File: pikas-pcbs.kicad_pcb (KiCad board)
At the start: 2 copper layers, 84.1 x 43.7 mm, 24 parts, among them SW1 SW_Push, U1 ATmega32U4-AU, Y1 16MHz

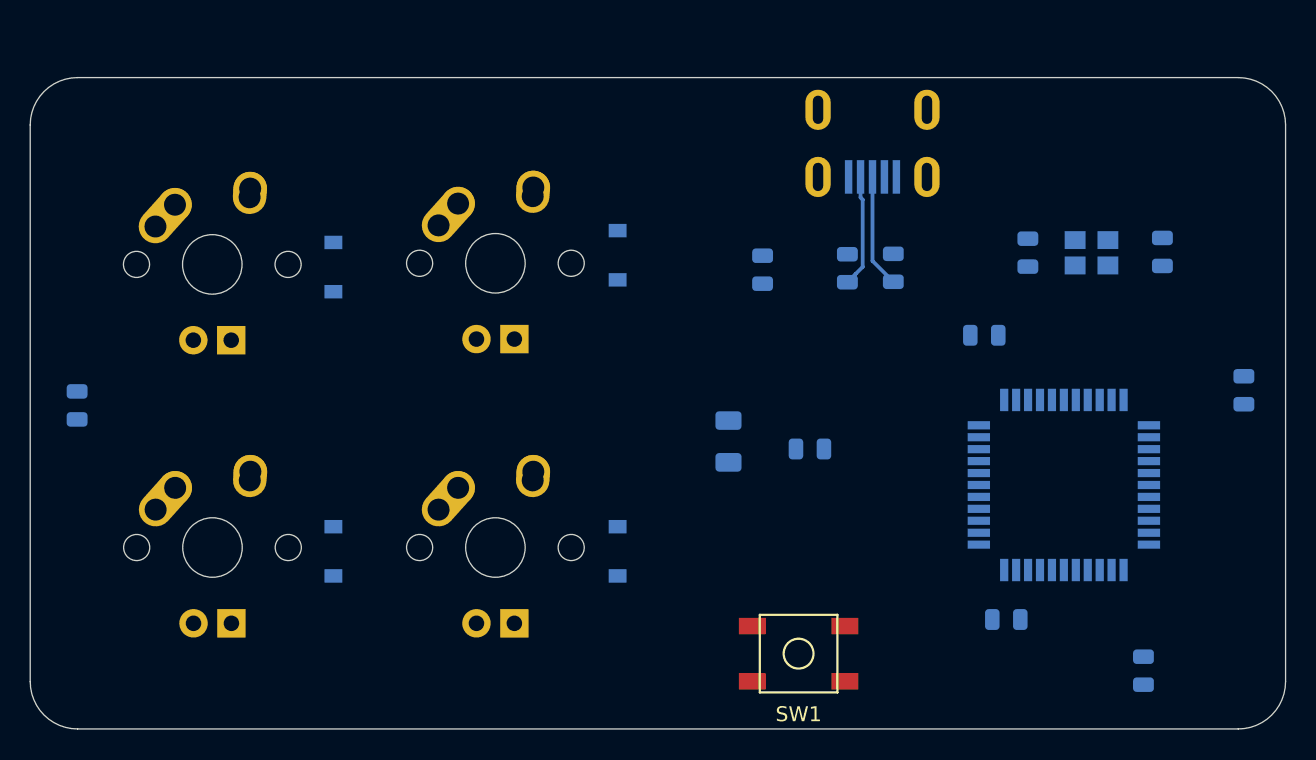
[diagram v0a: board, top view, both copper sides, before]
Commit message: SQUARE!!!
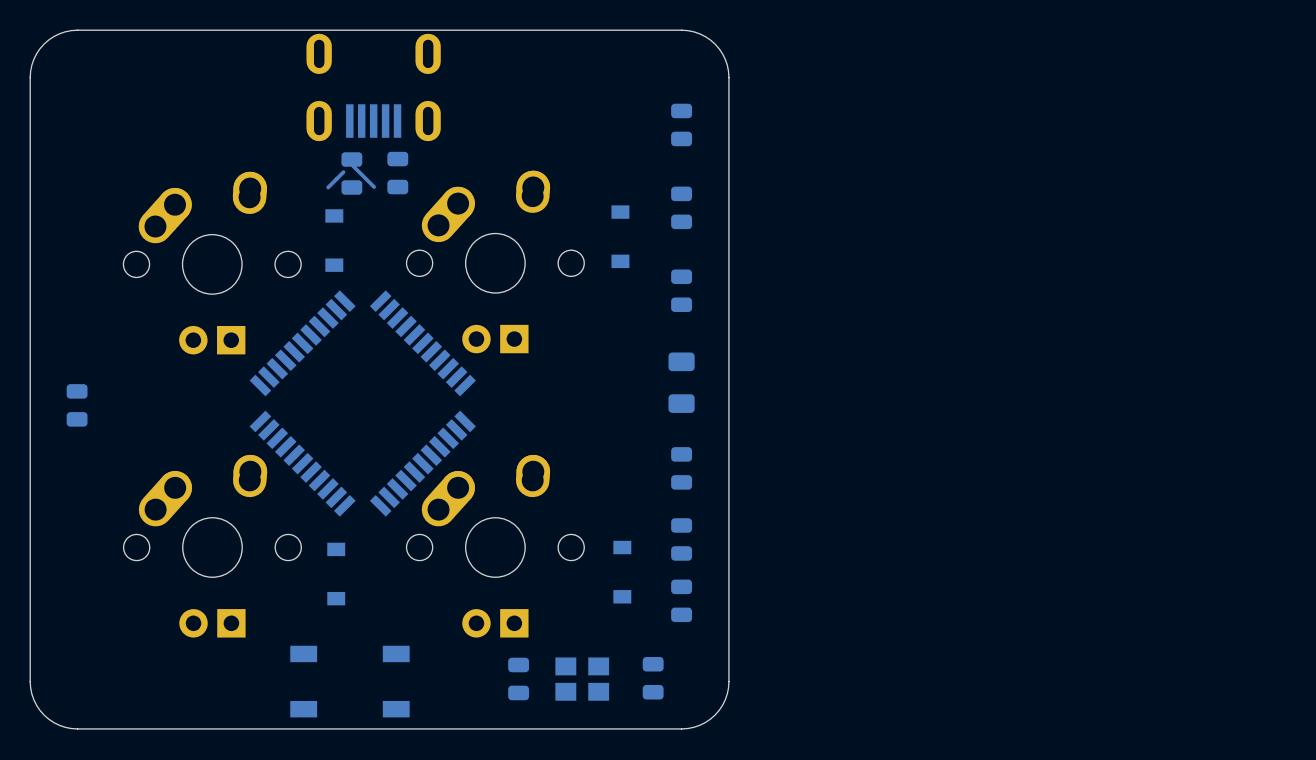
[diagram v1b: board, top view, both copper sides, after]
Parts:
- D1, D2, D3, D4: value D_Small -> SOD_123
- SW1: moved to B.Cu
- moved U1 47.3 mm to (96.9, 63.1), turned to 45 degrees
- moved C1 44.5 mm to (116.4, 81.5)
- moved C2 44.5 mm to (107.3, 81.6)
- moved Y1 44.5 mm to (111.6, 81.6)
- moved C5 38.3 mm to (118.3, 55.6), turned to 270 degrees
- moved R2 33.8 mm to (99.3, 47.7)
- moved R1 33.8 mm to (96.2, 47.7)
- moved USB1 33.6 mm to (97.6, 39.7)
- moved R4 31.3 mm to (118.3, 76.3)
- moved SW1 30.1 mm to (96.0, 81.8)
- moved C6 24.7 mm to (118.3, 44.5), turned to 270 degrees
- moved C7 22.4 mm to (118.3, 72.2), turned to 270 degrees
- moved C3 8.70 mm to (118.3, 67.5), turned to 270 degrees
- moved R3 6.83 mm to (118.3, 50.0), turned to 270 degrees
- moved F1 5.04 mm to (118.3, 61.7), turned to 270 degrees
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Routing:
- net D+: track 7.61 -> 0.00 mm
- net D-: track 7.54 -> 1.45 mm
- net Net-(R1-Pad2): track 0.00 -> 1.98 mm
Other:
- board size 84.1 x 43.7 mm -> 46.8 x 46.8 mm
